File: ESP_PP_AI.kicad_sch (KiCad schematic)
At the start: 46 parts, among them IC1 LM66200DRLR, J1 TYPE-C-31-M-12, J2 BAT_IN, Q1 AO3401A, SW1 SWITCH, SW2 EN, SW3 BOOT, U1 XC6206P282MR, U2 MCP23017-E/SO-ND, U3 TPS63020DSJR, U4 MCP73831-2ACI_MC, U5 USBLC6-2SC6, U6 ESP32-S3-WROOM-1, U7 XC6206P122MR

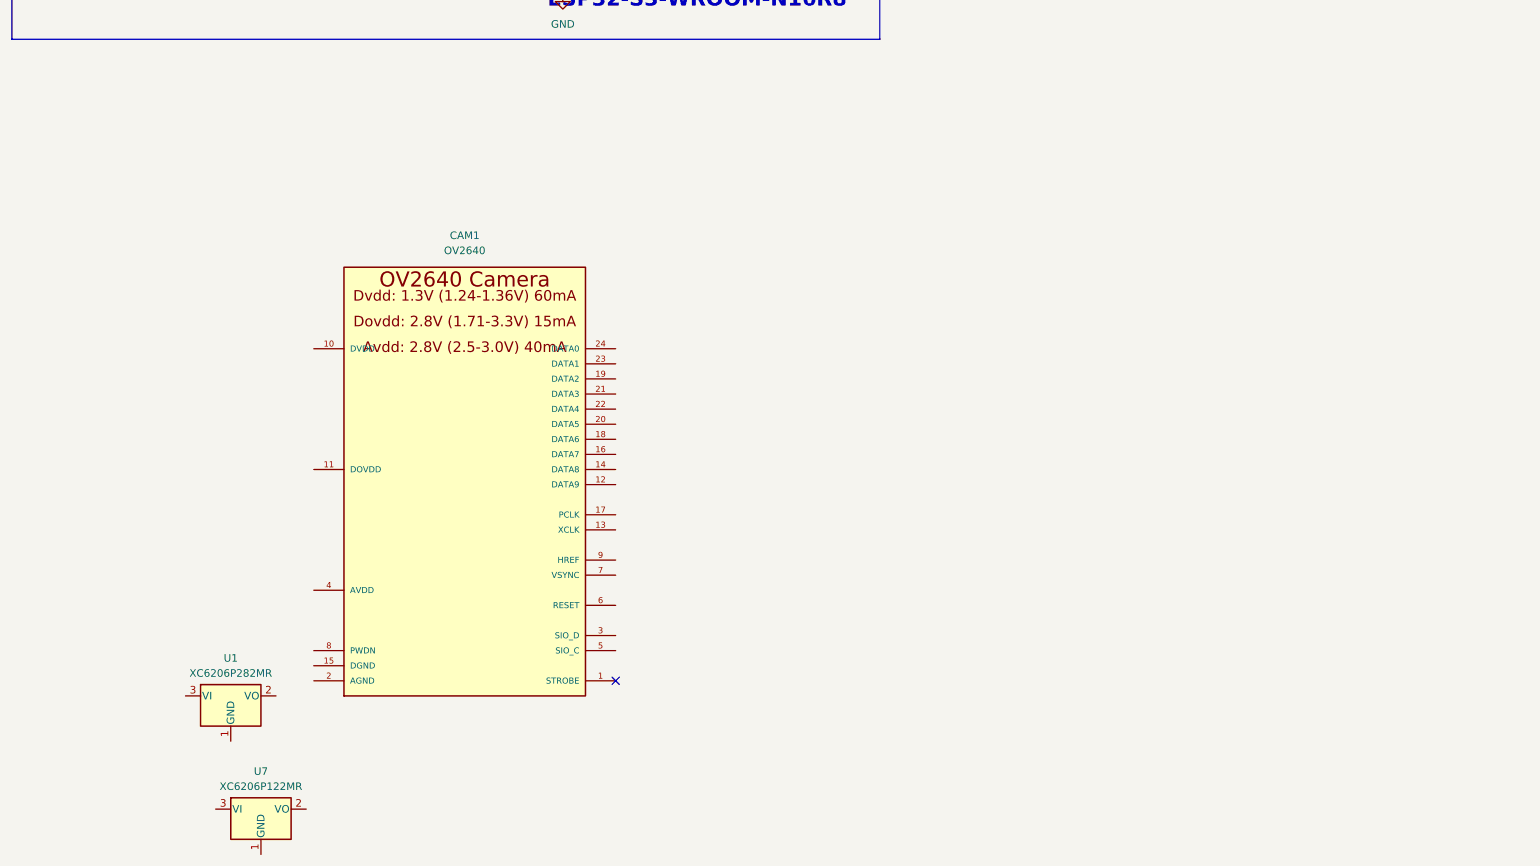
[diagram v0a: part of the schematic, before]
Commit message: added_cam
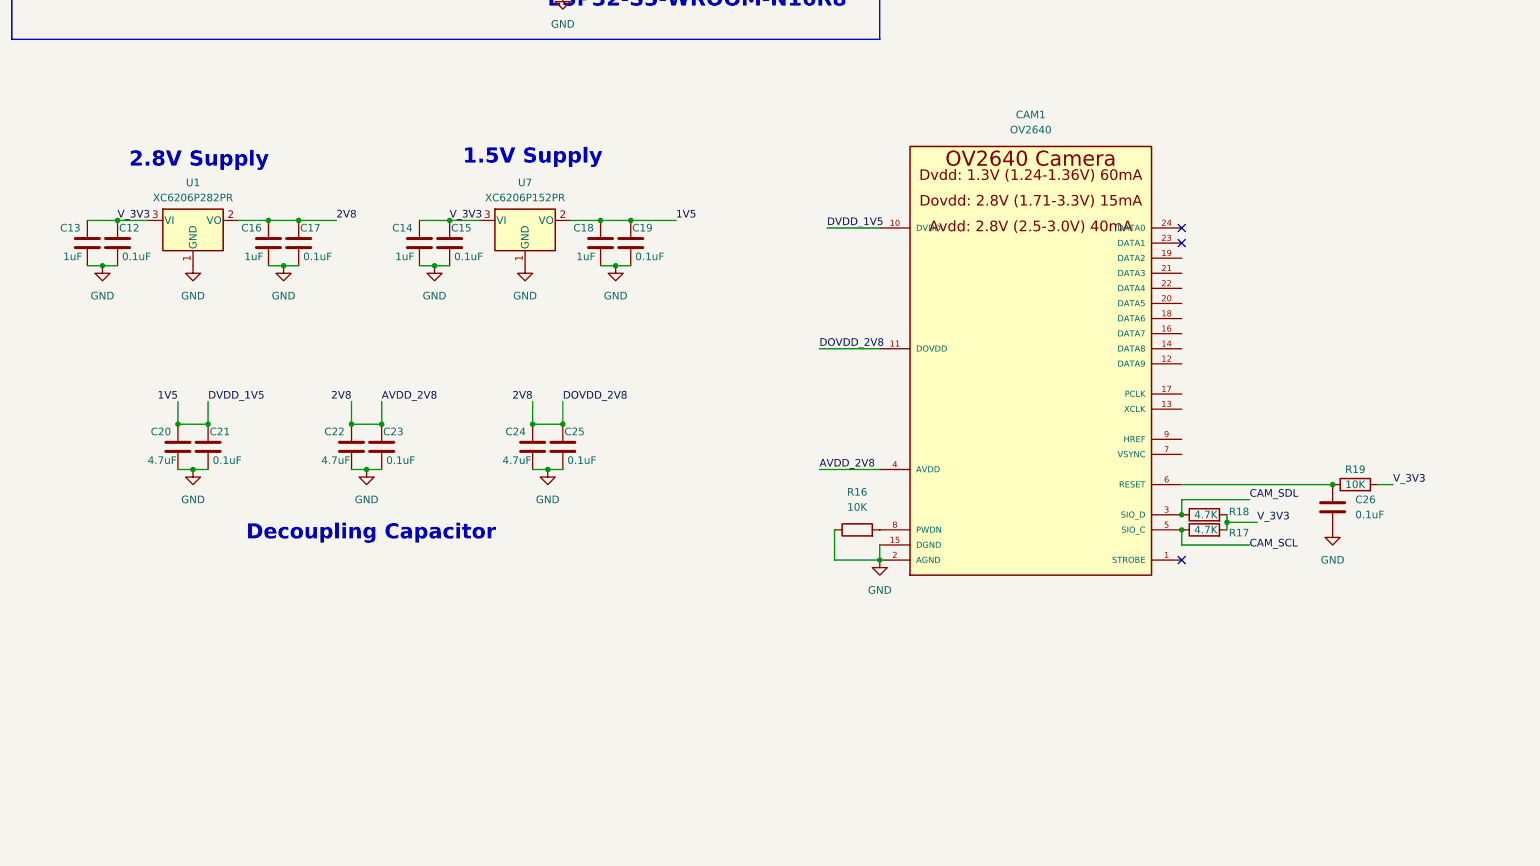
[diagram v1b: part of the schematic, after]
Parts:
- added C12, C15, C17, C19, C21, C23, C25, C26: 0.1uF, symbol Device:C
- added C13, C14, C16, C18: 1uF, symbol Device:C
- added C20, C22, C24: 4.7uF, symbol Device:C
- added R16, R19: 10K, symbol Device:R
- added R17, R18: 4.7K, symbol Device:R
- U1: value XC6206P282MR -> XC6206P282PR
- U7: value XC6206P122MR -> XC6206P152PR
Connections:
- net GND: now also CAM1.15 (DGND), CAM1.2 (AGND), CAM1.MT1 (DGND), CAM1.MT2 (DGND), U1.1 (GND), U7.1 (GND), C12.2, C13.2, C14.2, C15.2, C16.2, C17.2, C18.2, C19.2, C20.2, C21.2, C22.2, C23.2, C24.2, C25.2, C26.1, R16.1
- net V_3V3: now also U1.3 (VI), U7.3 (VI), C12.1, C13.1, C14.1, C15.1, R17.2, R18.2, R19.2
- net 2V8: now reaches U1.2 (VO)
- net 2V8: now also CAM1.11 (DOVDD), CAM1.4 (AVDD), C16.1, C17.1, C22.1, C23.1, C24.1, C25.1
- net 1V5: now reaches CAM1.10 (DVDD)
- net 1V5: now also U7.2 (VO), C18.1, C19.1, C20.1, C21.1
- net CAM_SDL: now reaches CAM1.3 (SIO_D)
- net CAM_SDL: now also R18.1
- net CAM_SCL: now reaches CAM1.5 (SIO_C)
- net CAM_SCL: now also R17.1
- net at CAM1.6 (RESET): now also C26.2, R19.1
- net at CAM1.8 (PWDN): now also R16.2
- no-connect marks 6 -> 8
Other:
- note added: "1.5V Supply"
- note added: "2.8V Supply"
- note added: "Decoupling Capacitor"
- moved on the sheet: CAM1, U1, U7

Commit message: fixxed camera
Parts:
- added C27: 15pF, symbol Device:C
- R17, R18: now not fitted
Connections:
- net GND: now also C27.2
- net IO16: now reaches CAM1.12 (DATA9)
- net IO16: now also U6.9 (IO16)
- net IO15: now reaches CAM1.13 (XCLK)
- net IO15: now also U6.8 (IO15)
- net IO17: now reaches CAM1.14 (DATA8)
- net IO17: now also U6.10 (IO17)
- net IO18: now reaches CAM1.16 (DATA7)
- net IO18: now also U6.11 (IO18)
- net IO13: now reaches CAM1.17 (PCLK)
- net IO13: now also U6.21 (IO13), C27.1
- net IO12: now reaches CAM1.18 (DATA6)
- net IO12: now also U6.20 (IO12)
- net IO11: now reaches CAM1.19 (DATA2)
- net IO11: now also U6.19 (IO11)
- net IO10: now reaches CAM1.20 (DATA5)
- net IO10: now also U6.18 (IO10)
- net IO9: now reaches CAM1.21 (DATA3)
- net IO9: now also U6.17 (IO9)
- net IO8: now reaches CAM1.22 (DATA4)
- net IO8: now also U6.12 (IO8)
- net IO6: now reaches CAM1.7 (VSYNC)
- net IO6: now also U6.6 (IO6)
- net IO7: now reaches CAM1.9 (HREF)
- net IO7: now also U6.7 (IO7)
- net GPIO14: now reaches U6.22 (IO14)
- net GPIO21: now reaches U6.23 (IO21)
- net GPIO47: now reaches U6.24 (IO47)
- net GPIO48: now reaches U6.25 (IO48)
- net GPIO38: now reaches U6.31 (IO38)
- net GPIO2: now reaches U6.38 (IO2)
- net GPIO1: now reaches U6.39 (IO1)
- net GPIO4: now reaches U6.4 (IO4)
- net GPIO5: now reaches U6.5 (IO5)
- no-connect marks 8 -> 17
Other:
- note added: "IOxx -> CAM GPIOxx -> DEVICE"
- note added: "JTAG"
- note added: "JTAG_STP"
- note added: "OV2640 Camera"
- note added: "OV2640 Camera and Supplies"
- note added: "STRP"
- note added: "UART"
- moved on the sheet: C12, C13, C14, C15, C16, C17, C18, C19, C20, C21, C22, C23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
